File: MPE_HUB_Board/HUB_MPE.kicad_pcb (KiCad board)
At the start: 4 copper layers, 130 x 116.7 mm, 242 parts, among them J1 Conn_01x09, J2 Conn_01x03, J3 Conn_01x06, J4 Conn_01x07, J5 Conn_01x05, J6 Conn_01x05, Q1 IRLML0100TRPBF, T1 H1102NLT, T2 H1102NLT, T3 H1102NLT, T4 H1102NLT, T6 H1102NLT, U1 K7803M-1000R3_C2916516, U10 MAX3485ESA, U2 RTL8305NB-VB-CG, U3 MAX3485ESA, U4 ESP32-S3-MINI-1-N4R2, U5 VND7050AJTR, U6 VND7050AJTR, U7 W5500, U8 MAX3485ESA, U9 ADS1015IDGSR, X1 25Mhz, X2 25MHz

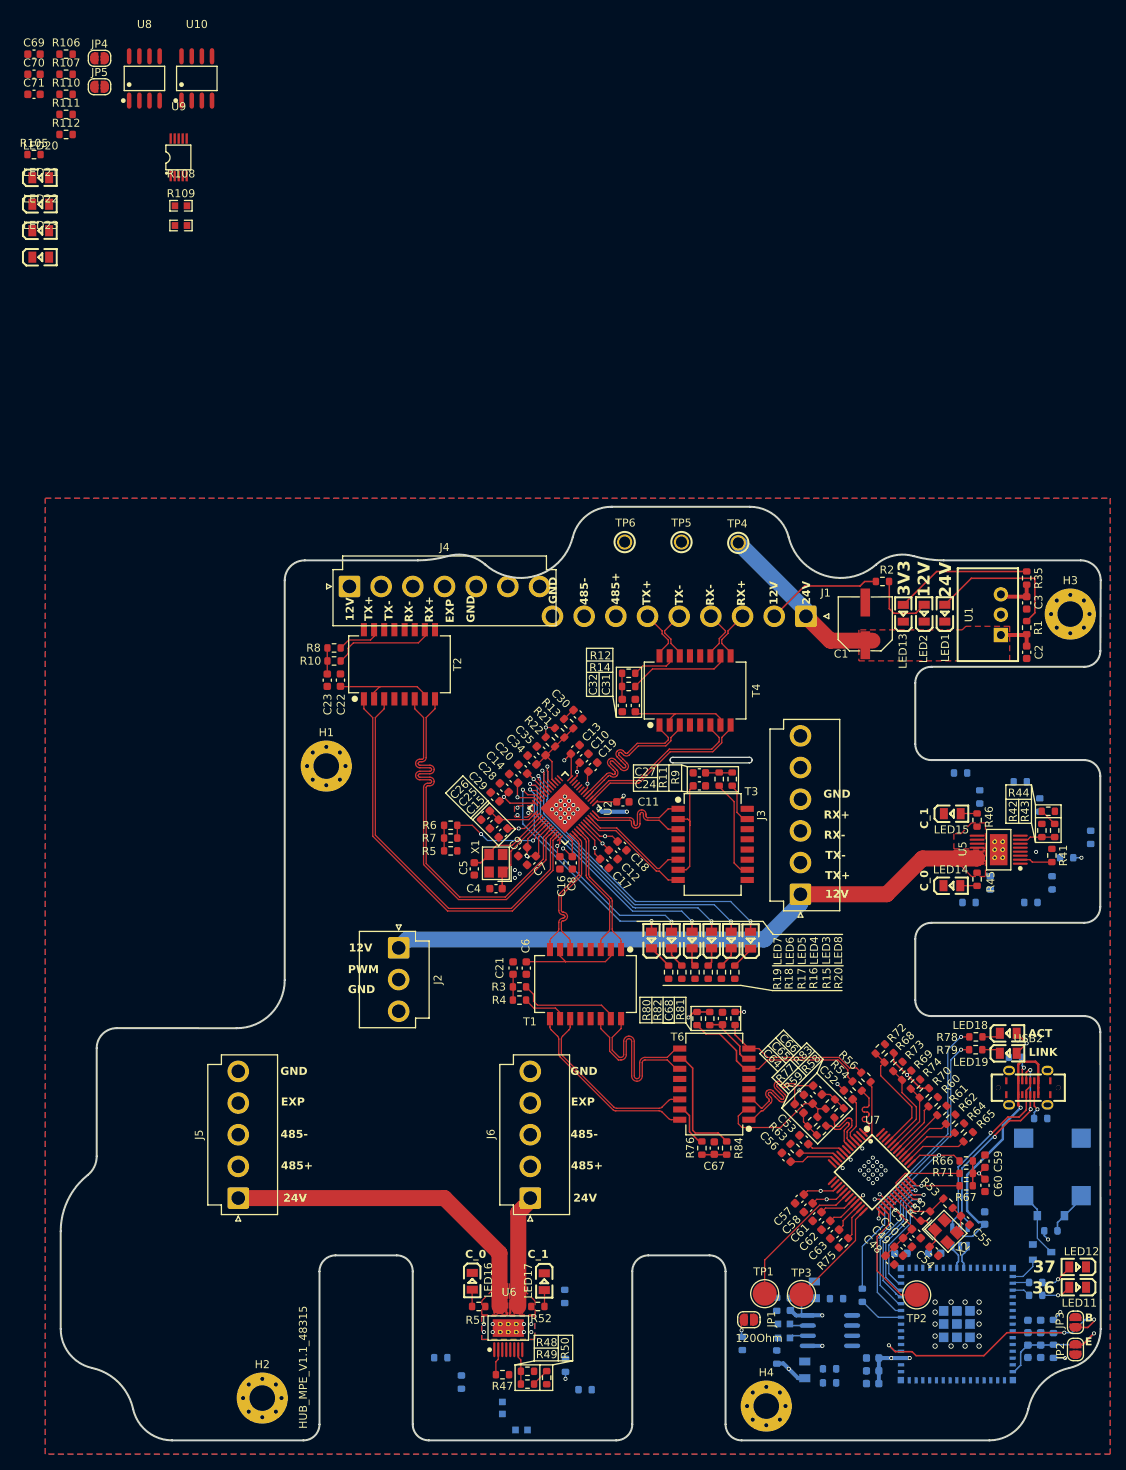
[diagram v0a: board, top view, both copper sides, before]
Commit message: HUB Hardware V1.1.0
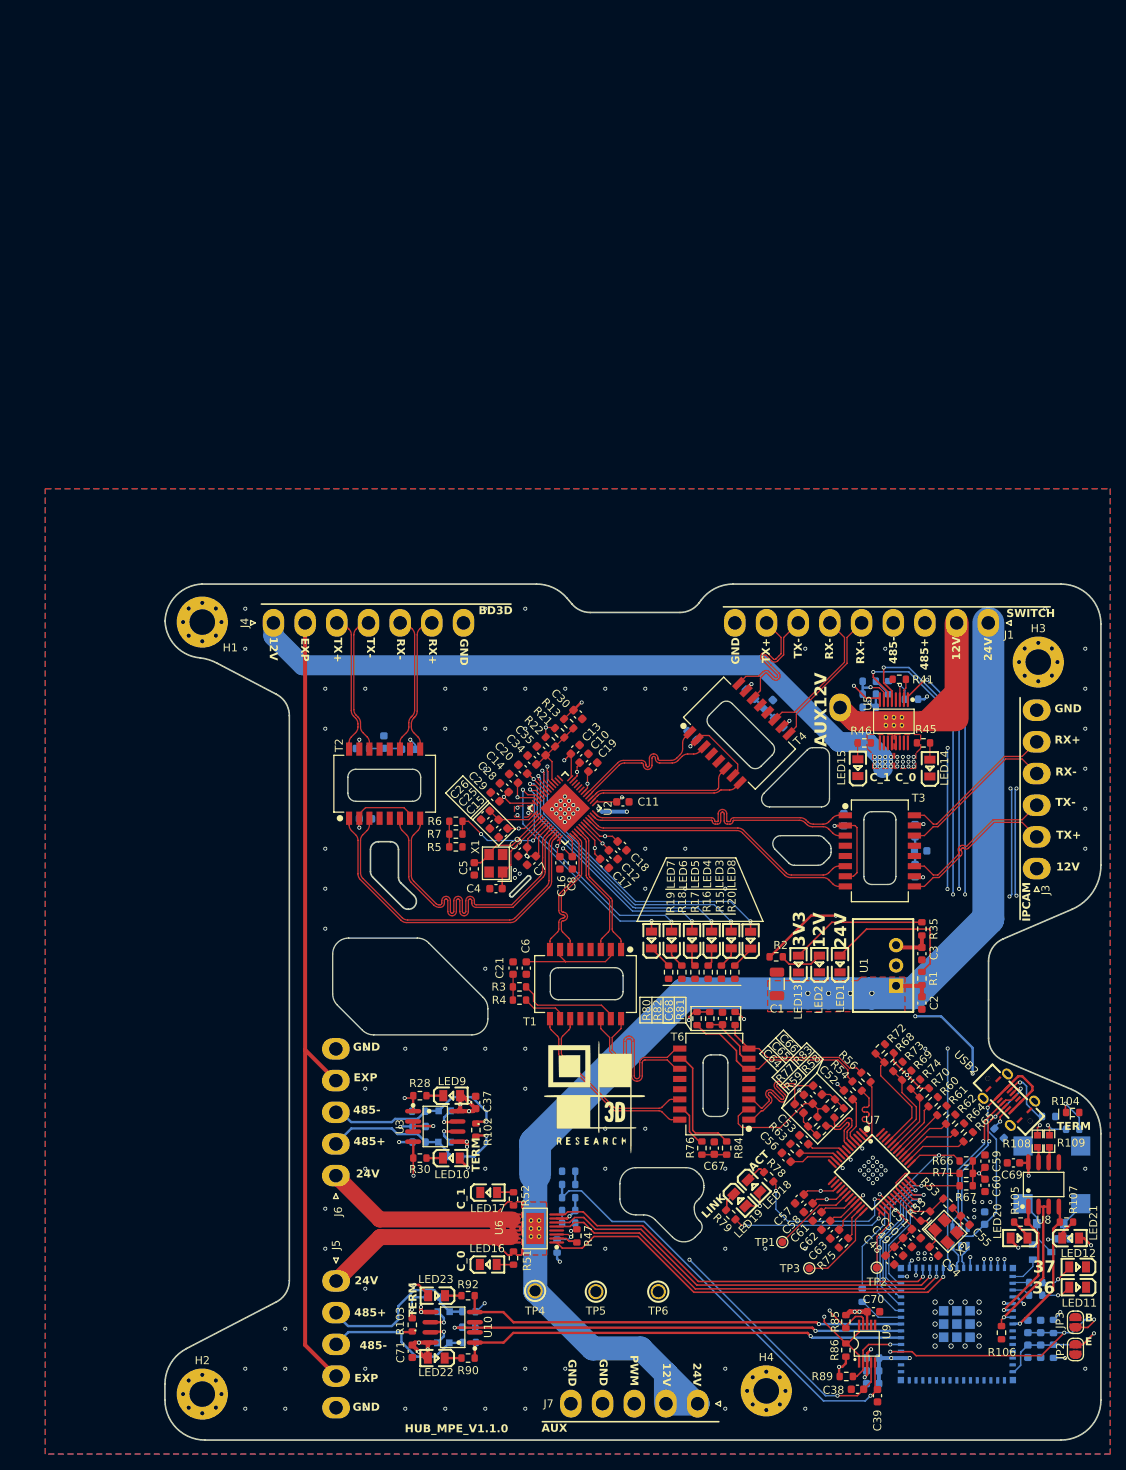
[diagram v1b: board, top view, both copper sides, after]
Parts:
- removed JP1, JP4, JP5: SolderJumper_2_Open, Jumper:SolderJumper-2_P1.3mm_Open_RoundedPad1.0x1.5mm
- removed R110, R112: 10K, Resistor_SMD:R_0603_1608Metric
- added G***: LOGO, LOGO, F.Cu at (95.4, 94.9)
- added J7: Conn_01x05, Connector_JST:JST_VH_B5P-VH-B_1x05_P3.96mm_Vertical, F.Cu at (108.4, 133.7)
- added R102: 0, Resistor_SMD:R_0603_1608Metric, F.Cu at (80.7, 99.5)
- added R103: 0, Resistor_SMD:R_0603_1608Metric, F.Cu at (72.8, 123.8)
- added R104: 0, Resistor_SMD:R_0603_1608Metric, F.Cu at (155.3, 97.3)
- C1: value 33uF 35V -> 22uF 35V; footprint easyeda2kicad:CAP-SMD_BD6.3-L6.6-W6.6-FD -> Capacitor_SMD:C_1206_3216Metric
- C22, C23, C24, C27, C31, C32, R10, R11, R111, R12, R14, R42, R43, R44, R48, R49, R50, R8, R9: moved to B.Cu
- C37, C38, C39, LED10, LED9, R28, R30, R85, R86, R89, R90, R92, U3: moved to F.Cu
- J2: value Conn_01x03 -> Conn_01x01_Pin; footprint Connector_JST:JST_VH_B3P-VH_1x03_P3.96mm_Vertical -> Connector_Wire:SolderWire-0.75sqmm_1x01_D1.25mm_OD3.5mm
- TP1, TP2, TP3: footprint TestPoint:TestPoint_Pad_D3.0mm -> TestPoint:TestPoint_Pad_D1.0mm
- U1: value K7803M-1000R3_C2916516 -> K7803M-1000R3
- moved R106 198.0 mm to (146.4, 124.8), turned to -90 degrees
- moved R107 190.3 mm to (154.5, 111.0), turned to 180 degrees
- moved C70 186.9 mm to (130.4, 122.2), turned to 180 degrees
- moved C69 184.9 mm to (147.9, 103.6)
- moved LED21 182.4 mm to (155.1, 113.0)
- moved R105 181.7 mm to (148.8, 111.0)
- moved LED20 180.3 mm to (148.6, 113.0), turned to 180 degrees
- moved R111 178.7 mm to (155.3, 99.4), turned to 180 degrees
- moved U8 178.2 mm to (151.7, 106.3)
- moved U9 171.5 mm to (129.6, 126.2)
- moved C71 164.1 mm to (72.8, 127.2), turned to 90 degrees
- moved U10 159.3 mm to (77.8, 124.2), turned to 90 degrees
- moved R108 158.5 mm to (150.9, 100.9), turned to 90 degrees
- moved R109 157.8 mm to (152.4, 100.9), turned to 90 degrees
- moved LED22 149.3 mm to (75.8, 128.0), turned to 180 degrees
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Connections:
- J1 pad 3: /ETH_ROV_RX+ -> /485_ROV+
- J1 pad 4: /ETH_ROV_RX- -> /485_ROV-
- J1 pad 5: /ETH_ROV_TX- -> /ETH_ROV_RX+
- J1 pad 6: /ETH_ROV_TX+ -> /ETH_ROV_RX-
- J1 pad 7: /485_ROV+ -> /ETH_ROV_TX-
- J1 pad 8: /485_ROV- -> /ETH_ROV_TX+
- J2 pad 1: /+12V_LIGHT_IPCAM -> +12V
- J4 pad 2: /ETH_BD3D_TX+ -> /EXPOSURE
- J4 pad 3: /ETH_BD3D_TX- -> /ETH_BD3D_TX+
- J4 pad 4: /ETH_BD3D_RX- -> /ETH_BD3D_TX-
- J4 pad 5: /ETH_BD3D_RX+ -> /ETH_BD3D_RX-
- J4 pad 6: /EXPOSURE -> /ETH_BD3D_RX+
- R86 pad 2: /MCU_ESP32/SDA -> /MCU_ESP32/SCL
- U4 pad 18: /MCU_ESP32/24V_EC_0 -> /MCU_ESP32/24V_EC_1
- U4 pad 19: /MCU_ESP32/24V_SEL_0 -> /MCU_ESP32/24V_SEL_1
- U4 pad 20: /MCU_ESP32/24V_SEL_1 -> /MCU_ESP32/24V_SEL_0
- U4 pad 21: /MCU_ESP32/24V_EC_1 -> /MCU_ESP32/24V_EC_0
- U4 pad 6: /MCU_ESP32/TX2_485_LED1 -> /MCU_ESP32/RX2_485_LED1
- U4 pad 8: /MCU_ESP32/RX2_485_LED1 -> /MCU_ESP32/TX2_485_LED1
- U5 pad : (no net) -> +12V
- U6 pad : (no net) -> +24V
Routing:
- net +24V: track 26.9 -> 162.1 mm, vias 8 -> 4
- net /+12V_MULTISENSE: track 0.00 -> 122.8 mm, vias 0 -> 3
- net /RESET_SWITCH: track 1.58 -> 108.4 mm, vias 0 -> 4
- net /MCU_ESP32/12V_SEL_1: track 0.00 -> 90.9 mm, vias 0 -> 3
- net /MCU_ESP32/12V_SEL_0: track 0.00 -> 88.9 mm, vias 0 -> 3
- net /+12V_BD3D: track 0.00 -> 85.4 mm, vias 0 -> 12
- net /MCU_ESP32/12V_EC_1: track 0.00 -> 84.0 mm, vias 0 -> 4
- net /MCU_ESP32/RX3_485_LED2: track 0.00 -> 81.7 mm, vias 0 -> 2
- net /MCU_ESP32/12V_EC_0: track 0.00 -> 79.0 mm, vias 0 -> 3
- net /485_ROV+: track 0.00 -> 78.0 mm, vias 0 -> 3
- net /MCU_ESP32/R/W_485_LED2: track 0.00 -> 77.0 mm, vias 0 -> 2
- net /485_ROV-: track 0.00 -> 75.2 mm, vias 0 -> 3
- net /MCU_ESP32/TX3_485_LED2: track 0.00 -> 71.9 mm, vias 0 -> 2
- net /EXPOSURE: track 36.5 -> 101.9 mm
- net /PWM_LIGHT: track 0.00 -> 62.2 mm, vias 0 -> 1
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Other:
- board size 130 x 116.7 mm -> 117 x 107 mm
- board text added: ". TERM"
- board text added: "AUX"
- board text added: "AUX12V"
- board text added: "BD3D"
- board text added: "D"
- board text added: "HUB_MPE_V1.1.0"
- board text added: "IPCAM"
- board text added: "R"
- board text added: "SWITCH"
- board text added: "TERM ."
- board text added: "| | TERM"
- board text removed: "120Ohm"
- board text removed: "HUB_MPE_V1.1_48315"
